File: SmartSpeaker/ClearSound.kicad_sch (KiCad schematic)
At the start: 29 parts

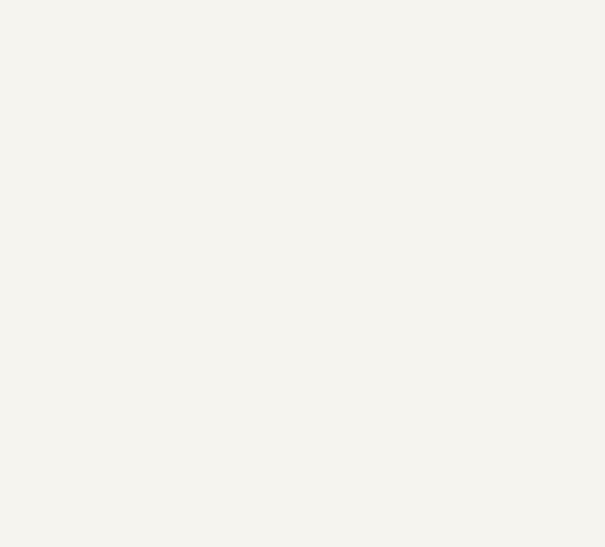
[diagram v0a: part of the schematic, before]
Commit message: add component
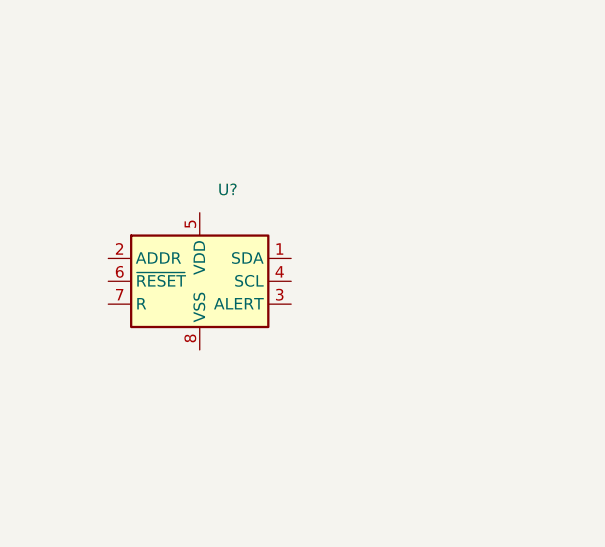
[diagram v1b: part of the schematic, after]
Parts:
- added U?: (no value), symbol Sensor_Humidity:SHT30A-DIS
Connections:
- new net: U?.8 (VSS), U?.9 (VSS)
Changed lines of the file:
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@@
     (pin "1")
+  )
+  (symbol (lib_id "Sensor_Humidity:SHT30A-DIS") (at 58.42 58.42 0) (unit 1)
+    (in_bom yes) (on_board yes) (fields_autoplaced)
+    (property "Reference" "U?" (id 0) (at 60.4394 48.26 0)
+      (effects (font (size 1.27 1.27)) (justify left))
+    )
+    (property "Value" "" (id 1) (at 60.4394 50.8 0)
+      (effects (font (size 1.27 1.27)) (justify left))
+    )
+    (property "Footprint" "" (id 2) (at 58.42 57.15 0)
+      (effects (font (size 1.27 1.27)) hide)
+    )
+    (property "Datasheet" "https://www.sensirion.com/fileadmin/user_upload/customers/sensirion/Dokumente/2_Humidity_Sensors/Datasheets/Sensirion_Humidity_Sensors_SHT3xA_Datasheet.pdf" (id 3) (at 58.42 57.15 0)
+      (effects (font (size 1.27 1.27)) hide)
+    )
+    (pin "1")
+    (pin "2")
+    (pin "3")
+    (pin "4")
+    (pin "5")
+    (pin "6")
+    (pin "7")
+    (pin "8")
+    (pin "9")
   )
   (symbol (lib_id "Device:L_Iron") (at 520.7 76.2 90) (unit 1)
@@
       (reference "R?") (unit 1) (value "51k Ω") (footprint "")
     )
-  )
+    (path "/60c7fec2-c4fb-4b6e-8f3b-028c31d0244e"
+      (reference "U?") (unit 1) (value "SHT30A-DIS") (footprint "Sensor_Humidity:Sensirion_DFN-8-1EP_2.5x2.5mm_P0.5mm_EP1.1x1.7mm")
+    )
+  )

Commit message: Remove redundant
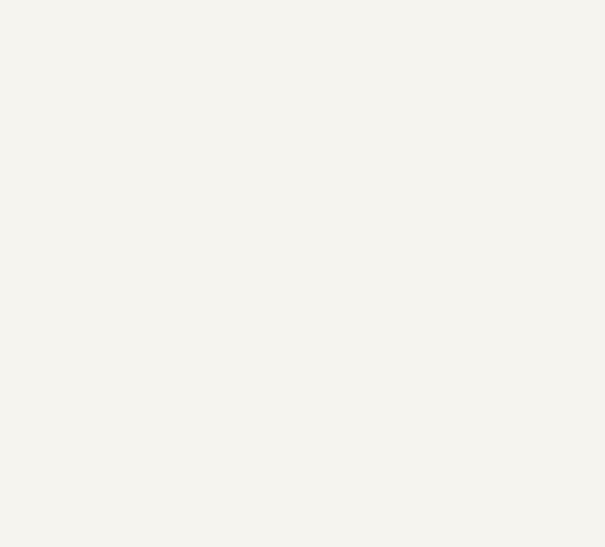
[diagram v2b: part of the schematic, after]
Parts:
- removed U?: (no value), symbol Sensor_Humidity:SHT30A-DIS
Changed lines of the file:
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@@
     (pin "1")
-  )
-  (symbol (lib_id "Sensor_Humidity:SHT30A-DIS") (at 58.42 58.42 0) (unit 1)
-    (in_bom yes) (on_board yes) (fields_autoplaced)
-    (property "Reference" "U?" (id 0) (at 60.4394 48.26 0)
-      (effects (font (size 1.27 1.27)) (justify left))
-    )
-    (property "Value" "" (id 1) (at 60.4394 50.8 0)
-      (effects (font (size 1.27 1.27)) (justify left))
-    )
-    (property "Footprint" "" (id 2) (at 58.42 57.15 0)
-      (effects (font (size 1.27 1.27)) hide)
-    )
-    (property "Datasheet" "https://www.sensirion.com/fileadmin/user_upload/customers/sensirion/Dokumente/2_Humidity_Sensors/Datasheets/Sensirion_Humidity_Sensors_SHT3xA_Datasheet.pdf" (id 3) (at 58.42 57.15 0)
-      (effects (font (size 1.27 1.27)) hide)
-    )
-    (pin "1")
-    (pin "2")
-    (pin "3")
-    (pin "4")
-    (pin "5")
-    (pin "6")
-    (pin "7")
-    (pin "8")
-    (pin "9")
   )
   (symbol (lib_id "Device:L_Iron") (at 520.7 76.2 90) (unit 1)
@@
       (reference "R?") (unit 1) (value "51k Ω") (footprint "")
     )
-    (path "/60c7fec2-c4fb-4b6e-8f3b-028c31d0244e"
-      (reference "U?") (unit 1) (value "SHT30A-DIS") (footprint "Sensor_Humidity:Sensirion_DFN-8-1EP_2.5x2.5mm_P0.5mm_EP1.1x1.7mm")
-    )
-  )
+  )
